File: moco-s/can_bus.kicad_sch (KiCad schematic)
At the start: 21 parts, among them J8 Conn_02x02_Top_Bottom, J9 Conn_02x02_Top_Bottom, U4 MCP2515-xST, U5 TJA1051T-3, Y3 8MHz

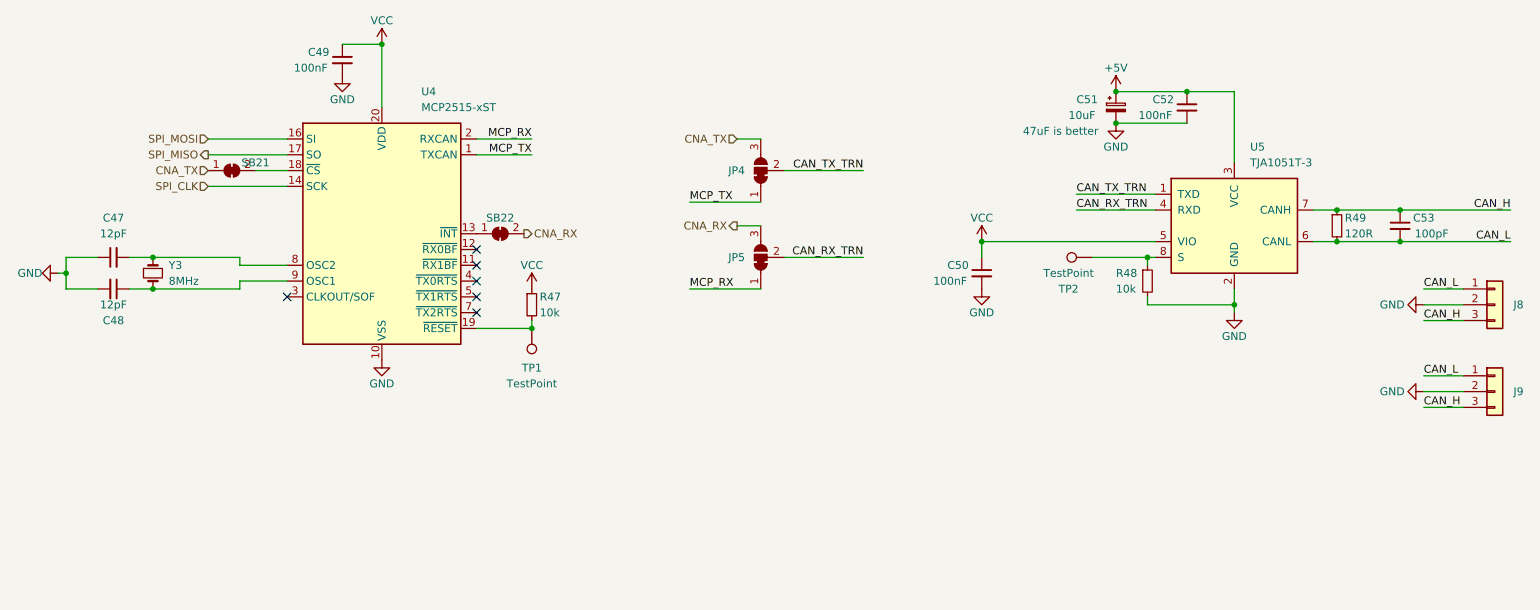
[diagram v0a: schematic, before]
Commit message: Update layout
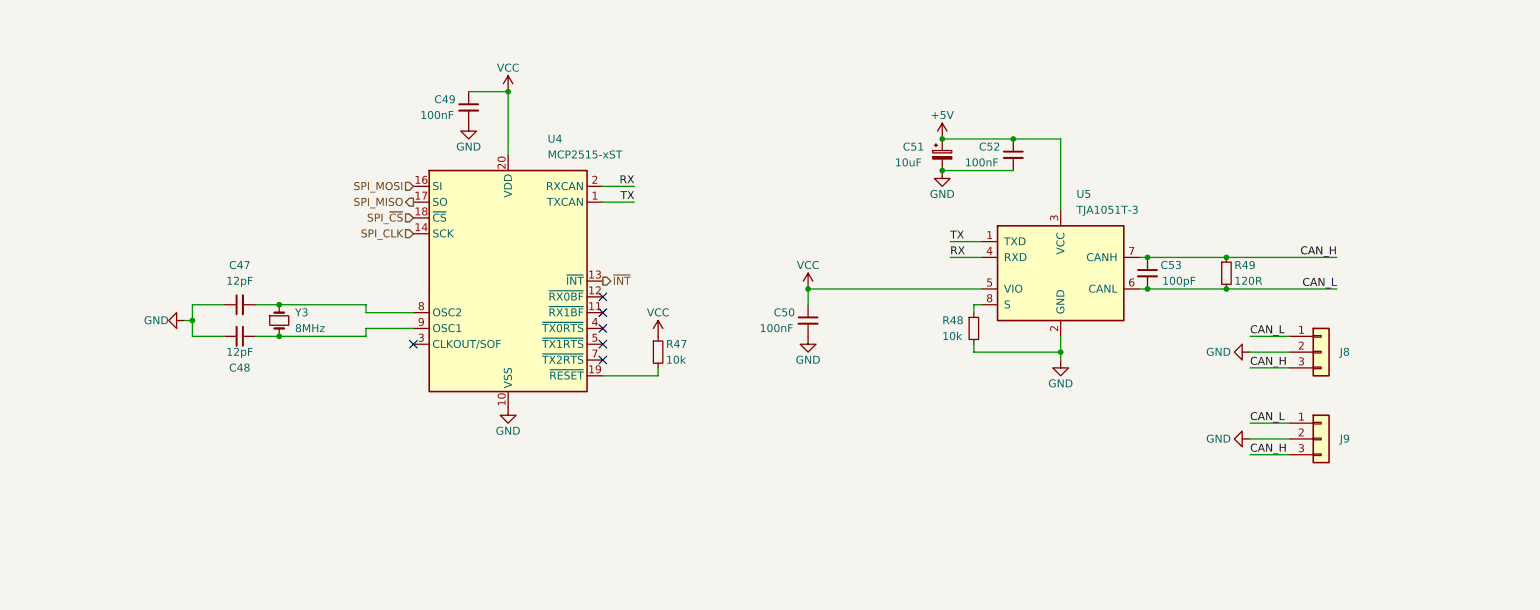
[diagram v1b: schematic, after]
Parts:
- removed JP4, JP5: SolderJumper_3_Bridged12, Jumper:SolderJumper-3_P1.3mm_Bridged12_RoundedPad1.0x1.5mm_NumberLabels, symbol Jumper:SolderJumper_3_Bridged12
- removed SB21, SB22: SolderJumper_2_Bridged, Jumper:SolderJumper-2_P1.3mm_Bridged_RoundedPad1.0x1.5mm, symbol Jumper:SolderJumper_2_Bridged
- removed TP1, TP2: TestPoint, TestPoint:TestPoint_Pad_D2.0mm, symbol Connector:TestPoint
- C51: Note 47uF is better -> (none)
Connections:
- net MCP_RX is gone; now on net RX: U4.2 (RXCAN)
- net MCP_TX is gone; now on net TX: U4.1 (TXCAN)
- net ~{INT}: now reaches U4.13 (~{INT})
- net SPI_~{CS}: now reaches U4.18 (~{CS})
- net CAN_RX_TRN renamed RX
- net CAN_TX_TRN renamed TX
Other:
- moved on the sheet: C47, C48, C49, C50, C51, C52, C53, J8, J9, R47, R48, R49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

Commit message: Comp MoCo-S
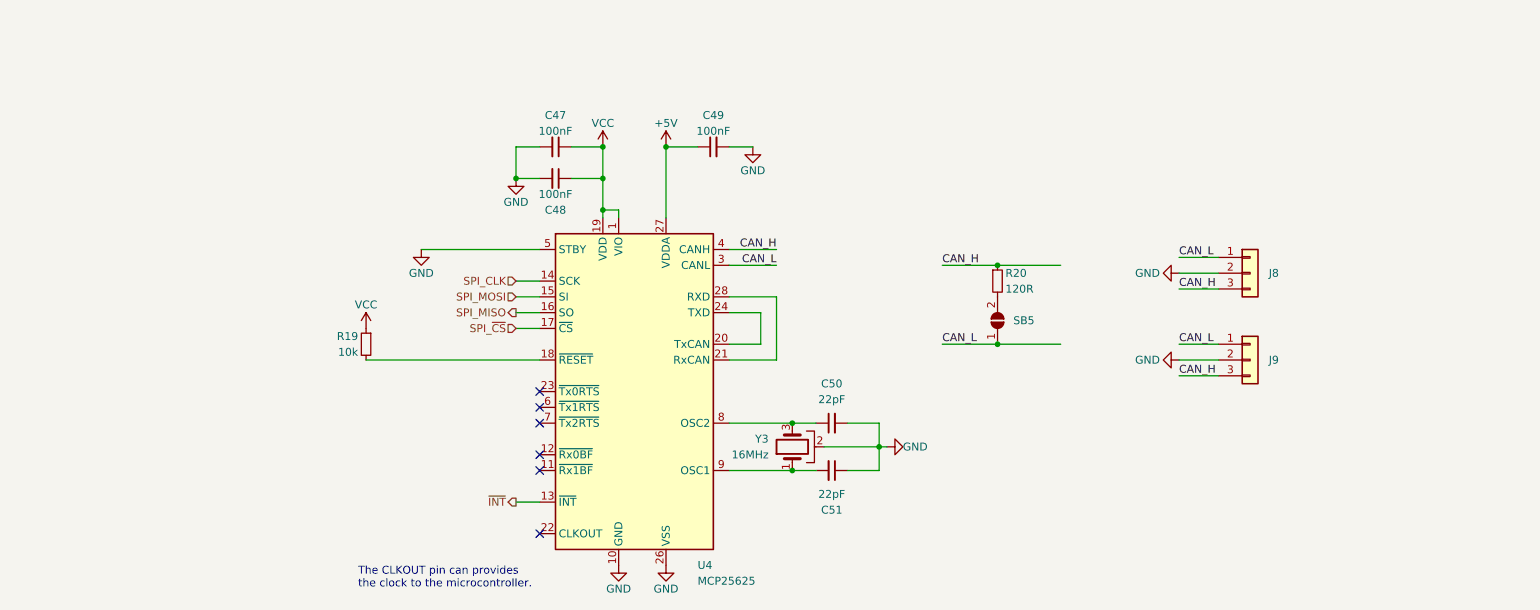
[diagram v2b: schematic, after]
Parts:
- removed C51: 10uF, Capacitor_Tantalum_SMD:CP_EIA-3216-18_Kemet-A, symbol Device:C_Polarized_Small
- removed C52: 100nF, Capacitor_SMD:C_0402_1005Metric, symbol Device:C_Small
- removed C53: 100pF, Capacitor_SMD:C_0402_1005Metric, symbol Device:C_Small
- removed R47, R48: 10k, Resistor_SMD:R_0402_1005Metric, symbol Device:R_Small
- removed R49: 120R, Resistor_SMD:R_0402_1005Metric, symbol Device:R_Small
- removed U4: MCP2515-xST, Package_SO:TSSOP-20_4.4x6.5mm_P0.65mm, symbol Interface_CAN_LIN:MCP2515-xST
- removed U5: TJA1051T-3, Package_SO:SOIC-8_3.9x4.9mm_P1.27mm, symbol Interface_CAN_LIN:TJA1051T-3
- removed Y3: 8MHz, Crystal:Crystal_SMD_Qantek_QC5CB-2Pin_5x3.2mm, symbol Device:Crystal_Small
- added C51: 22pF, Capacitor_SMD:C_0402_1005Metric, symbol Device:C_Small
- added R19: 10k, Resistor_SMD:R_0402_1005Metric, symbol Device:R_Small
- added R20: 120R, Resistor_SMD:R_0402_1005Metric, symbol Device:R_Small
- added SB5: SolderJumper_2_Open, Jumper:SolderJumper-2_P1.3mm_Open_TrianglePad1.0x1.5mm, symbol Jumper:SolderJumper_2_Open
- added U4: MCP25625, Package_DFN_QFN:QFN-28-1EP_6x6mm_P0.65mm_EP4.25x4.25mm, symbol Interface_CAN_LIN:MCP25625-x-SS
- added Y3: 16MHz, Crystal:Crystal_SMD_3225-4Pin_3.2x2.5mm, symbol Device:Crystal_GND2
- C47, C48: value 12pF -> 100nF; JLCPCB Part # (none) -> C1525; MFR.Part # (none) -> CL05B104KO5NNNC
- C50: value 100nF -> 22pF; JLCPCB Part # C1525 -> (none); MFR.Part # CL05B104KO5NNNC -> (none)
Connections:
- net +5V: now also C49.1, U4.27 (VDDA)
- net CAN_H: now also R20.1, U4.4 (CANH)
- net CAN_L: now also SB5.1 (A), U4.3 (CANL)
- net GND: now also C47.2, C51.1, U4.10 (GND), U4.26 (VSS), U4.5 (STBY), Y3.2; no longer C47.1
- net SPI_CLK: now also U4.14 (SCK)
- net SPI_MISO: now also U4.16 (SO)
- net SPI_MOSI: now also U4.15 (SI)
- net SPI_~{CS}: now also U4.17 (~{CS})
- net VCC: now also C47.1, C48.1, R19.1, U4.1 (VIO), U4.19 (VDD); no longer C49.1, C50.1
- net ~{INT}: now also U4.13 (~{INT})
- new net: C51.2, U4.9 (OSC1), Y3.1
- new net: C50.1, U4.8 (OSC2), Y3.3
- new net: R19.2, U4.18 (~{RESET})
- new net: U4.20 (TxCAN), U4.24 (TXD)
- new net: U4.21 (RxCAN), U4.28 (RXD)
- new net: R20.2, SB5.2 (B)
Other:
- note added: "The CLKOUT pin can provides the clock to the microcontroller."
- moved on the sheet: J8, J9
